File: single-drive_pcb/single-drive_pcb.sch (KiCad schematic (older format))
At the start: 29 parts

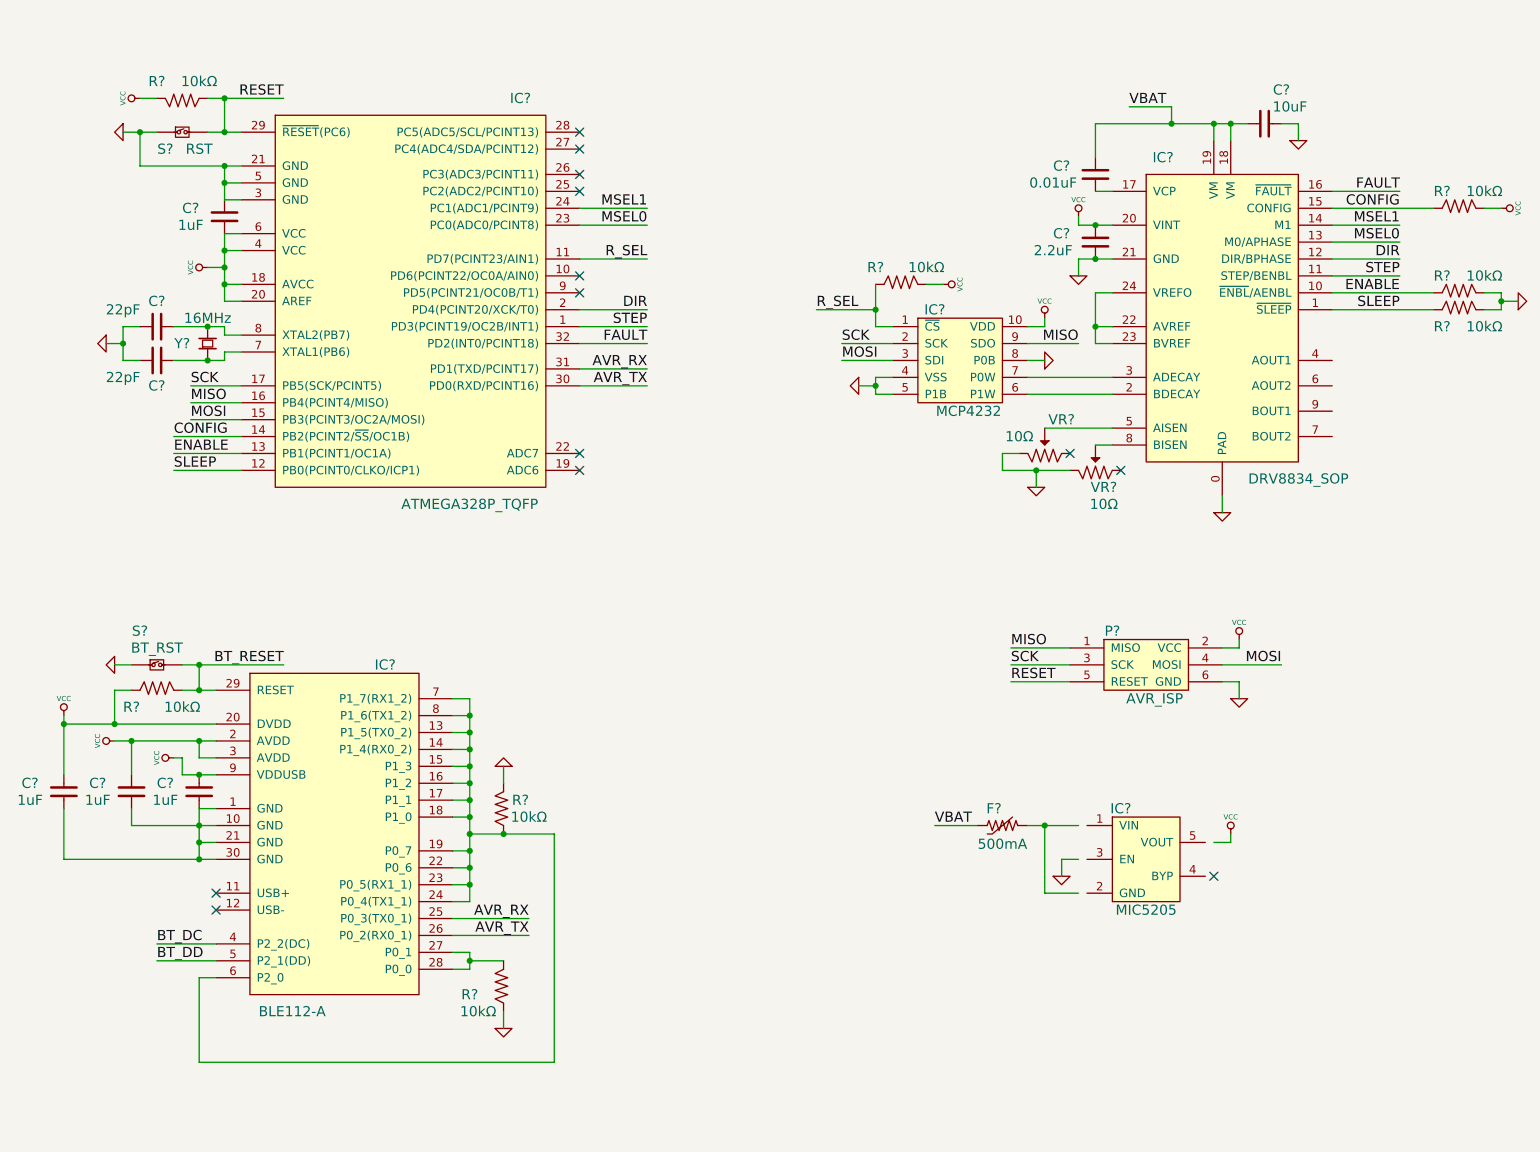
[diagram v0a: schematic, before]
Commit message: schematic is done (until I find problems); moving on to footprint assignment
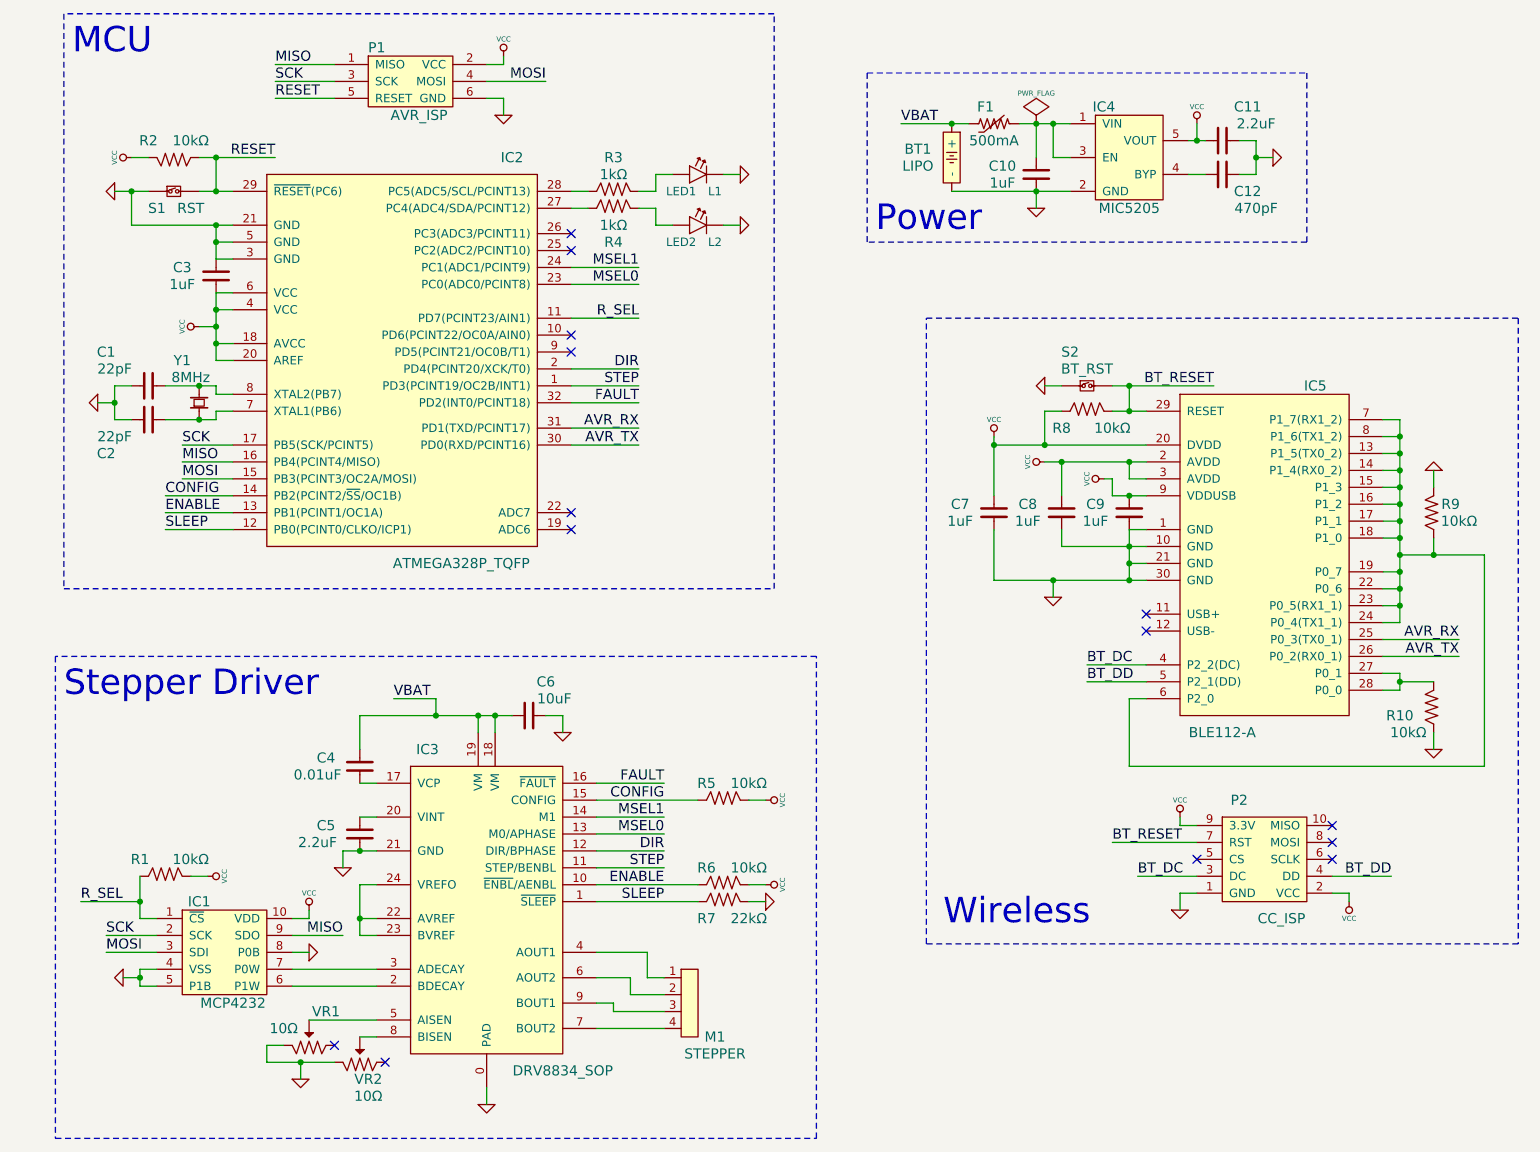
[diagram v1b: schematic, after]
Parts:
- added BT1: LIPO, symbol LIPO
- added C10: 1uF, ~, symbol C
- added C11: 2.2uF, ~, symbol C
- added C12: 470pF, ~, symbol C
- added LED1: L1, ~, symbol LED
- added LED2: L2, ~, symbol LED
- added M1: STEPPER, ~, symbol 4PIN_HEADER
- added P2: CC_ISP, ~, symbol CC_ISP
- added R3, R4: 1kΩ, ~, symbol R
- R7: renamed from R?; value 10kΩ -> 22kΩ
- Y1: renamed from Y?; value 16MHz -> 8MHz
- gave numbers to parts that had none: 27
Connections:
- net BT_DC: now also P2.3 (DC)
- net BT_DD: now also P2.4 (DD)
- net BT_RESET: now also P2.7 (RST)
- net GND: now also C7.1, C8.1, C9.1, IC4.2 (GND), IC5.1 (GND), IC5.10 (GND), IC5.21 (GND), IC5.30 (GND), BT1.2 (-), C10.1, C11.2, C12.2, LED1.1 (C), LED2.1 (C), P2.1 (GND); no longer R6.2
- net VBAT: now also BT1.1 (+)
- net VCC: now also IC4.5 (VOUT), R6.2, C11.1, P2.2 (VCC), P2.9 (3.3V); no longer C5.2, IC3.20 (VINT)
- net at IC3.4 (AOUT1): now also M1.1
- net at IC3.6 (AOUT2): now also M1.2
- net at IC3.7 (BOUT2): now also M1.4
- net at IC3.9 (BOUT1): now also M1.3
- net at IC2.27 (PC4(ADC4/SDA/PCINT12)): now also R4.1
- net at IC2.28 (PC5(ADC5/SCL/PCINT13)): now also R3.1
- net at IC4.1 (VIN): now also F1.2, IC4.3 (EN), C10.2
- net at IC4.4 (BYP): now also C12.1
- new net: C5.2, IC3.20 (VINT)
- new net: LED1.2 (A), R3.2
- new net: LED2.2 (A), R4.2
- no-connect marks 13 -> 14
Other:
- note added: "MCU"
- note added: "Power"
- note added: "Stepper Driver"
- note added: "Wireless"
- moved on the sheet: C1, C2, C3, C4, C5, C6, C7, C8, C9, F1, IC1, IC2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
